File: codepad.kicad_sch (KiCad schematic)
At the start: 37 parts, among them SW1 SW_Push, SW2 SW_Push, SW3 SW_Push, SW4 SW_Push, SW5 SW_Push, SW6 SW_Push, SW7 SW_Push, SW8 SW_Push, SW9 RotaryEncoder_Switch, U1 MOUDLE-SEEEDUINO-XIAO, U2 ER_OLEDM0.91_1x-I2C

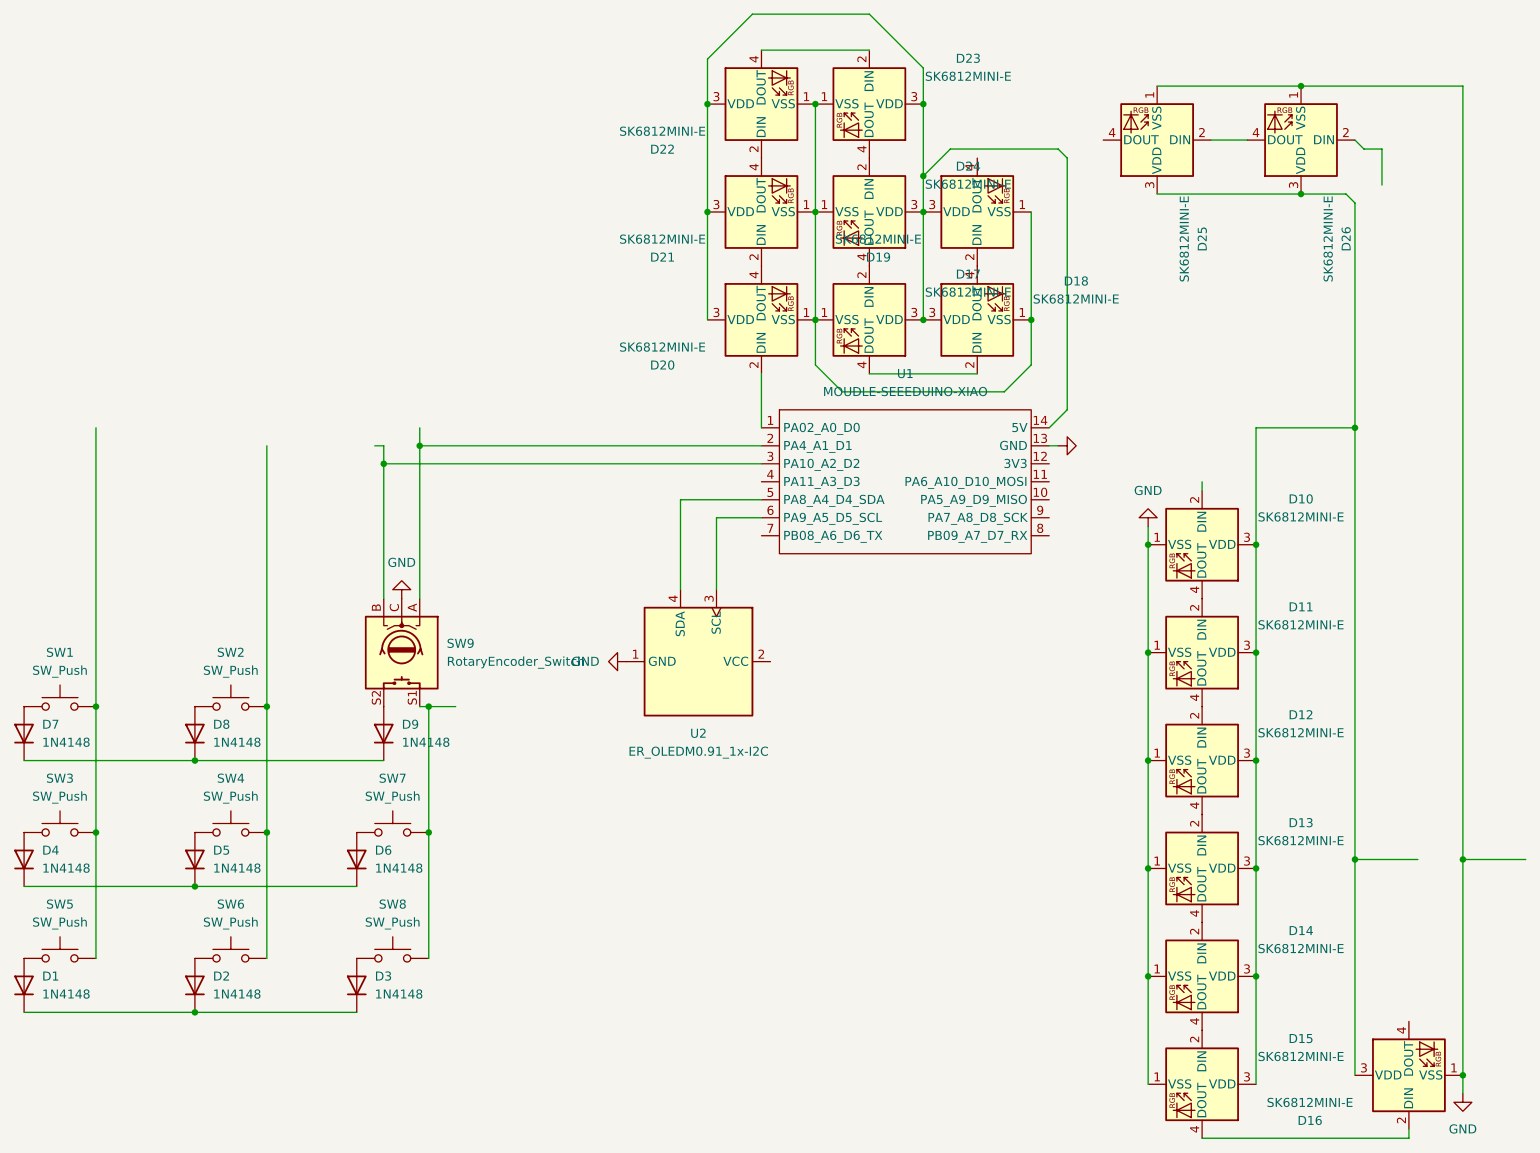
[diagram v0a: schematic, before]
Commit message: restart
working from start after watchinh a tutorial
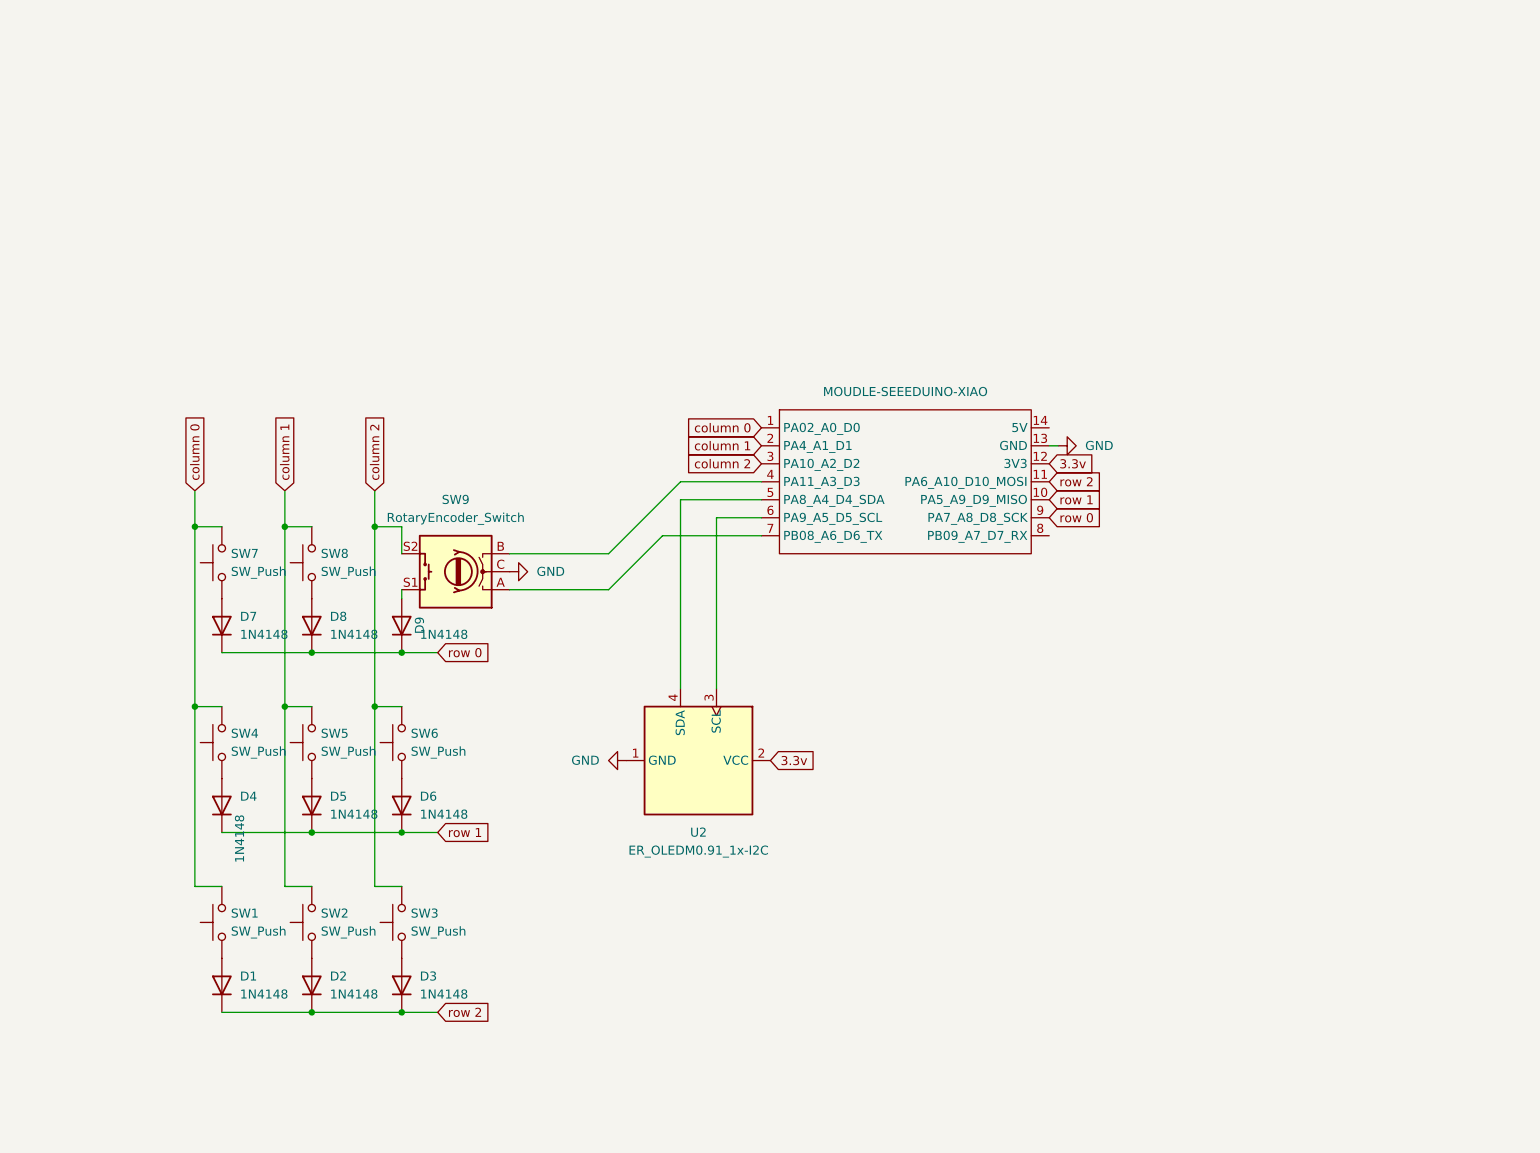
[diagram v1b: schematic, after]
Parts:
- removed D10, D11, D12, D13, D14, D15, D16, D17, D18, D19, D20, D21, D22, D23, D24, D25, D26: SK6812MINI-E, hackclub:SK6812MINI-E_fixed, symbol LED:SK6812MINI-E
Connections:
- net column 0: now reaches U1.1 (PA02_A0_D0)
- net column 0: now also SW1.2, SW4.2, SW7.2
- net row 1: now reaches U1.10 (PA5_A9_D9_MISO)
- net row 1: now also D4.1 (K), D5.1 (K), D6.1 (K)
- net row 2: now reaches U1.11 (PA6_A10_D10_MOSI)
- net row 2: now also D1.1 (K), D2.1 (K), D3.1 (K)
- net 3.3v: now reaches U1.12 (3V3)
- net 3.3v: now also U2.2 (VCC)
- net at SW9.A: now also U1.7 (PB08_A6_D6_TX); no longer U1.2 (PA4_A1_D1)
- net at SW9.B: now also U1.4 (PA11_A3_D3); no longer U1.3 (PA10_A2_D2)
- net row 0: now reaches U1.9 (PA7_A8_D8_SCK)
- net row 0: now also D7.1 (K), D8.1 (K), D9.1 (K)
- net at SW1.1: now also D1.2 (A); no longer D7.2 (A)
- net at D9.2 (A): now also SW9.S1; no longer SW9.S2
- net at D8.2 (A): now also SW8.1; no longer SW2.1
- net at SW5.1: now also D5.2 (A); no longer D1.2 (A)
- net at D3.2 (A): now also SW3.1; no longer SW8.1
- net at D4.2 (A): now also SW4.1; no longer SW3.1
- net at D6.2 (A): now also SW6.1; no longer SW7.1
- net at D2.2 (A): now also SW2.1; no longer SW6.1
- new net: D7.2 (A), SW7.1
- new net column 1: SW2.2, SW5.2, SW8.2, U1.2 (PA4_A1_D1)
- new net column 2: SW3.2, SW6.2, SW9.S2, U1.3 (PA10_A2_D2)
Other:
- moved on the sheet: U2
